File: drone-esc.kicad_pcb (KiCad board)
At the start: 4 copper layers, 34 x 34 mm, 237 parts, among them J1 SM08B-SRSS-TB_LF__SN_, Q1 IRLHS6242, Q10 IRLHS6242, Q11 IRLHS6242, Q12 IRLHS6242, Q13 IRLHS6242, Q14 IRLHS6242, Q15 IRLHS6242, Q16 IRLHS6242, Q17 IRLHS6242, Q18 IRLHS6242, Q19 IRLHS6242, Q2 IRLHS6242, Q20 IRLHS6242, Q21 IRLHS6242, Q22 IRLHS6242, Q23 IRLHS6242, Q24 IRLHS6242, Q3 IRLHS6242, Q4 IRLHS6242, Q5 IRLHS6242, Q6 IRLHS6242, Q7 IRLHS6242, Q8 IRLHS6242, Q9 IRLHS6242, U10 DGD05473FNQ-7, U11 DGD05473FNQ-7, U12 AT32F421G8U7, U13 DGD05473FNQ-7, U14 DGD05473FNQ-7, U15 DGD05473FNQ-7, U16 AT32F421G8U7, U17 DGD05473FNQ-7, U18 DGD05473FNQ-7, U19 DGD05473FNQ-7, U2 INA186A3IDCKR, U20 AT32F421G8U7, U3 TLV76733DRVR, U4 TPS61023DRLR, U5 AT32F421G8U7, U6 DGD05473FNQ-7, U7 DGD05473FNQ-7, U8 DGD05473FNQ-7, U9 DGD05473FNQ-7

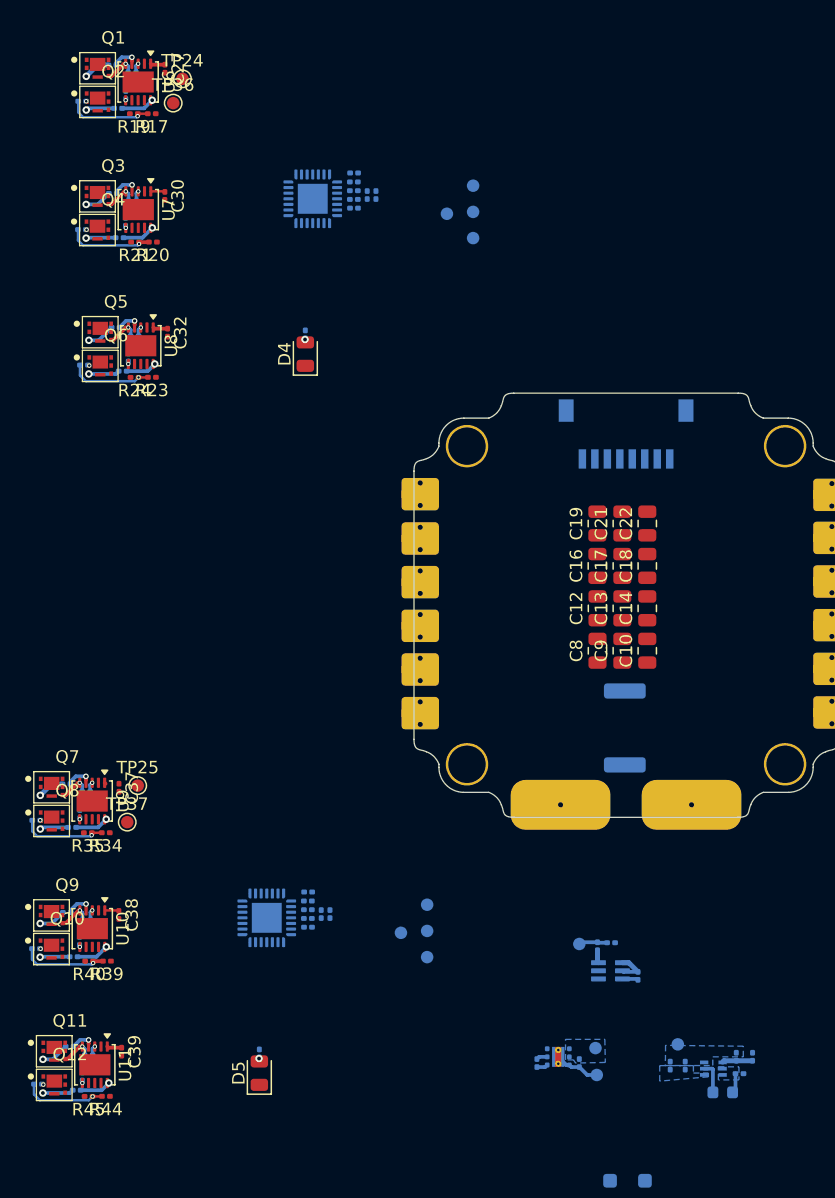
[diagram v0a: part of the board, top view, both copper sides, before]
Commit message: half placed
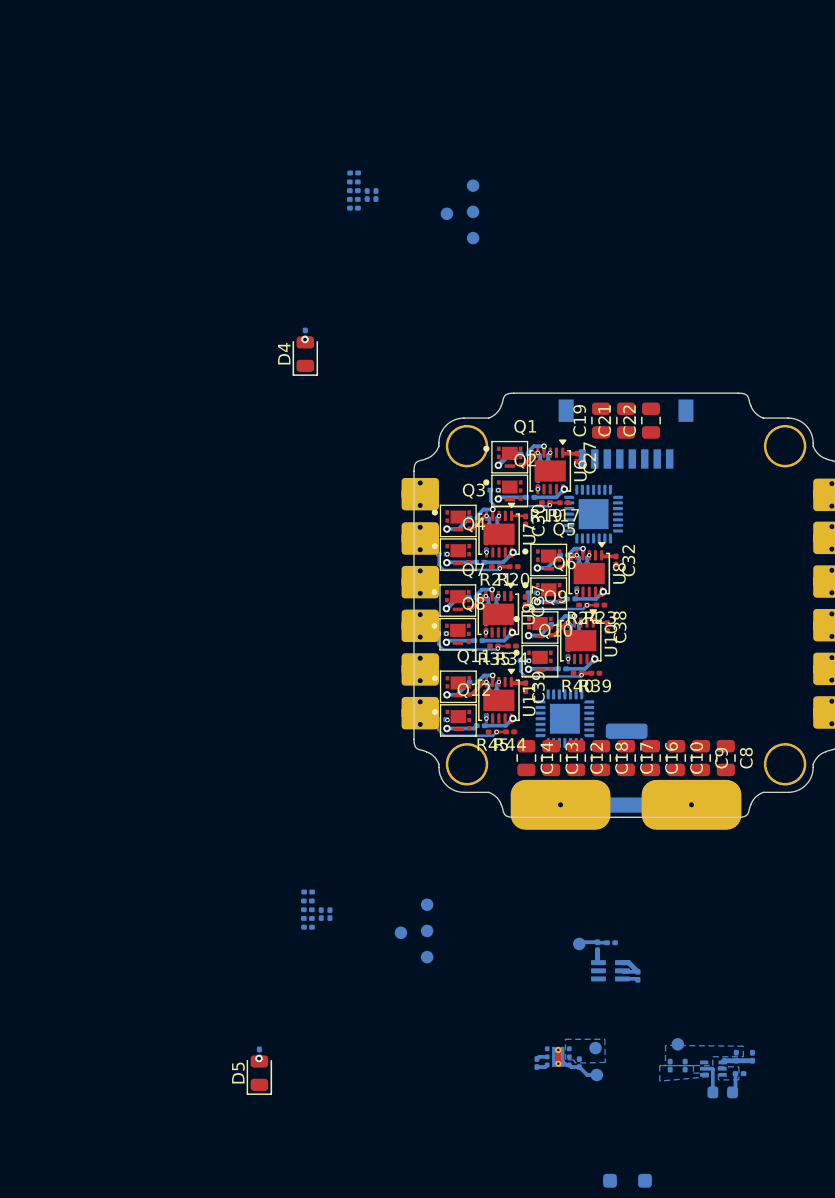
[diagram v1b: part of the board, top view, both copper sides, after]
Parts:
- removed TP24, TP25: GAH, TestPoint:TestPoint_Pad_D1.0mm
- removed TP36, TP37: GAL, TestPoint:TestPoint_Pad_D1.0mm
- moved Q10 45.5 mm to (138.1, 99.5)
- moved R36 45.5 mm to (139.3, 96.5)
- moved R37 45.5 mm to (139.9, 100.1)
- moved R40 45.5 mm to (141.1, 100.5)
- moved U10 45.5 mm to (141.4, 97.8)
- moved C34 45.5 mm to (140.9, 97.2)
- moved C38 45.5 mm to (143.5, 96.7)
- moved Q9 45.5 mm to (138.1, 96.8)
- moved R28 45.5 mm to (140.3, 98.8)
- moved R39 45.5 mm to (142.5, 100.5)
- moved R41 45.5 mm to (136.9, 99.5)
- moved Q1 45.4 mm to (135.7, 83.2)
- moved Q2 45.4 mm to (135.7, 85.8)
- moved U6 45.4 mm to (138.9, 84.2)
- moved R53 45.4 mm to (136.9, 82.9)
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
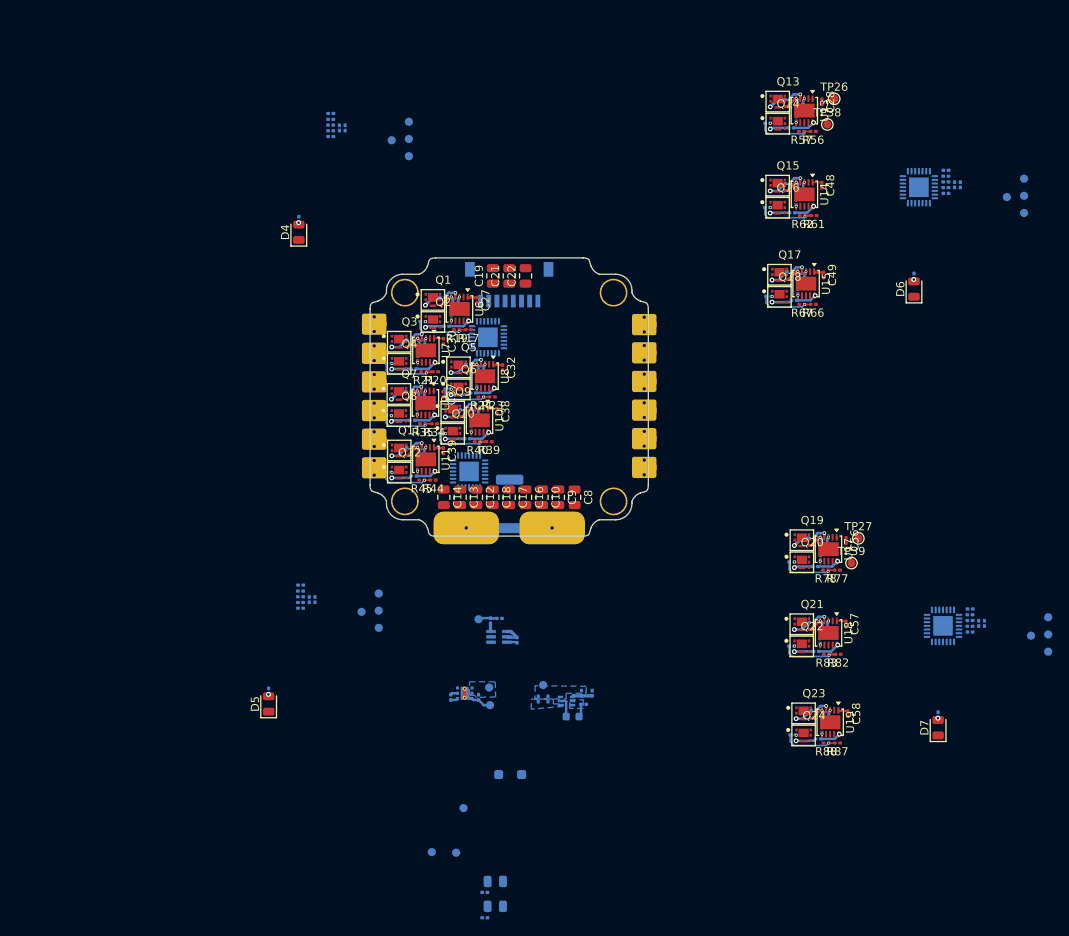
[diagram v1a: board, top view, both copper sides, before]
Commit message: main placing
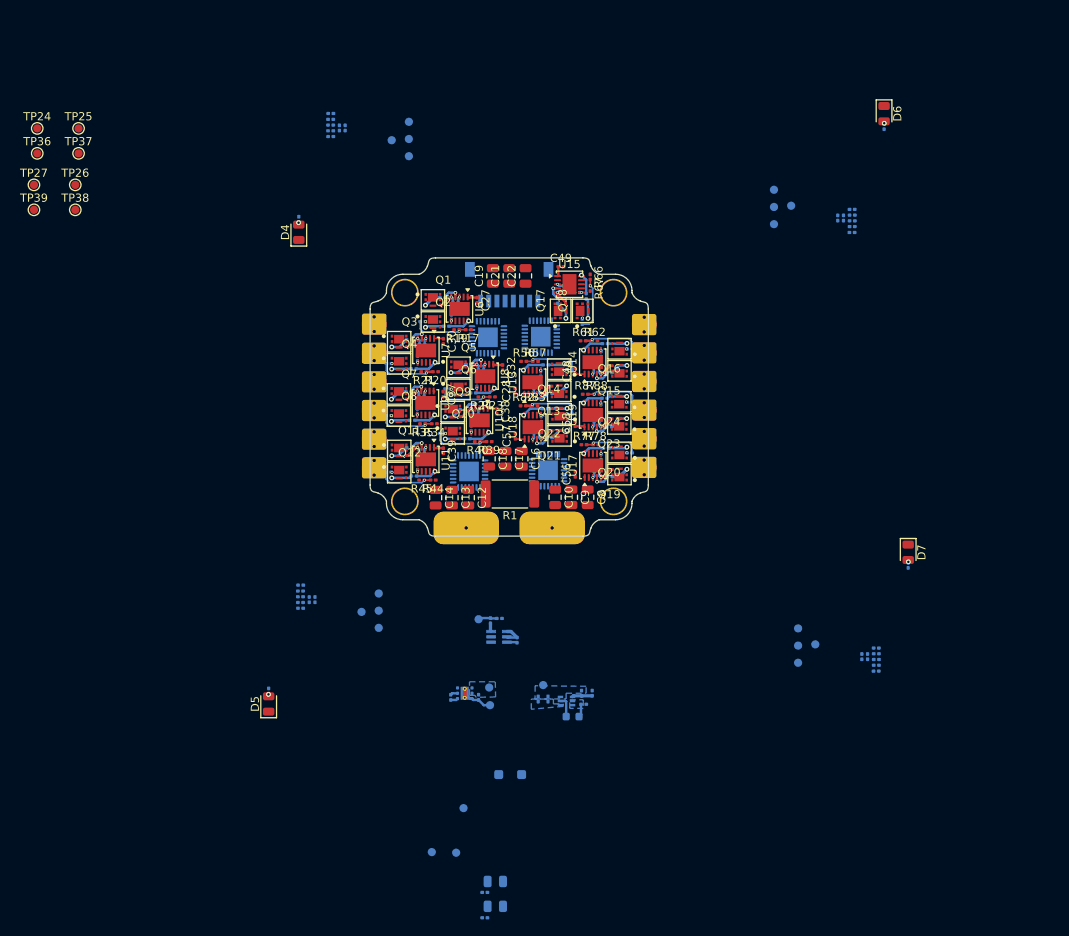
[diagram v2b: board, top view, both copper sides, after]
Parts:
- added TP24: GAH, TestPoint:TestPoint_Pad_D1.0mm, F.Cu at (87.3, 62.2)
- added TP25: GAH, TestPoint:TestPoint_Pad_D1.0mm, F.Cu at (92.4, 62.2)
- added TP36: GAL, TestPoint:TestPoint_Pad_D1.0mm, F.Cu at (87.3, 65.2)
- added TP37: GAL, TestPoint:TestPoint_Pad_D1.0mm, F.Cu at (92.4, 65.2)
- R1: moved to F.Cu
- moved TP27 109.6 mm to (86.9, 69.1)
- moved TP39 108.8 mm to (86.9, 72.1)
- moved TP26 93.3 mm to (92.0, 69.1)
- moved TP38 92.5 mm to (92.0, 72.1)
- moved R87 52.6 mm to (154.3, 94.7), turned to 0 degrees
- moved U20 51.9 mm to (149.8, 104.0), turned to 0 degrees
- moved C28 51.5 mm to (145.7, 94.3), turned to 90 degrees
- moved R88 51.0 mm to (155.7, 94.7), turned to 0 degrees
- moved U16 49.7 mm to (148.9, 87.6), turned to 0 degrees
- moved R86 49.1 mm to (156.7, 95.2), turned to 0 degrees
- moved R82 49.0 mm to (146.7, 96.1), turned to 0 degrees
- moved C58 48.7 mm to (153.1, 98.2), turned to 90 degrees
- moved R72 47.8 mm to (156.2, 96.2), turned to -90 degrees
- moved U19 47.5 mm to (155.2, 97.2), turned to 90 degrees
- moved C43 47.4 mm to (148.3, 93.9), turned to 0 degrees
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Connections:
- U1 pad 17: /ESC3/MotorA -> /ESC3/MotorC
- U1 pad 19: /ESC3/MotorC -> /ESC3/MotorA
- U1 pad 20: /ESC4/MotorA -> /ESC4/MotorC
- U1 pad 22: /ESC4/MotorC -> /ESC4/MotorA
